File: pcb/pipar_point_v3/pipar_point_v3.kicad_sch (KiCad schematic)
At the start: 3 parts

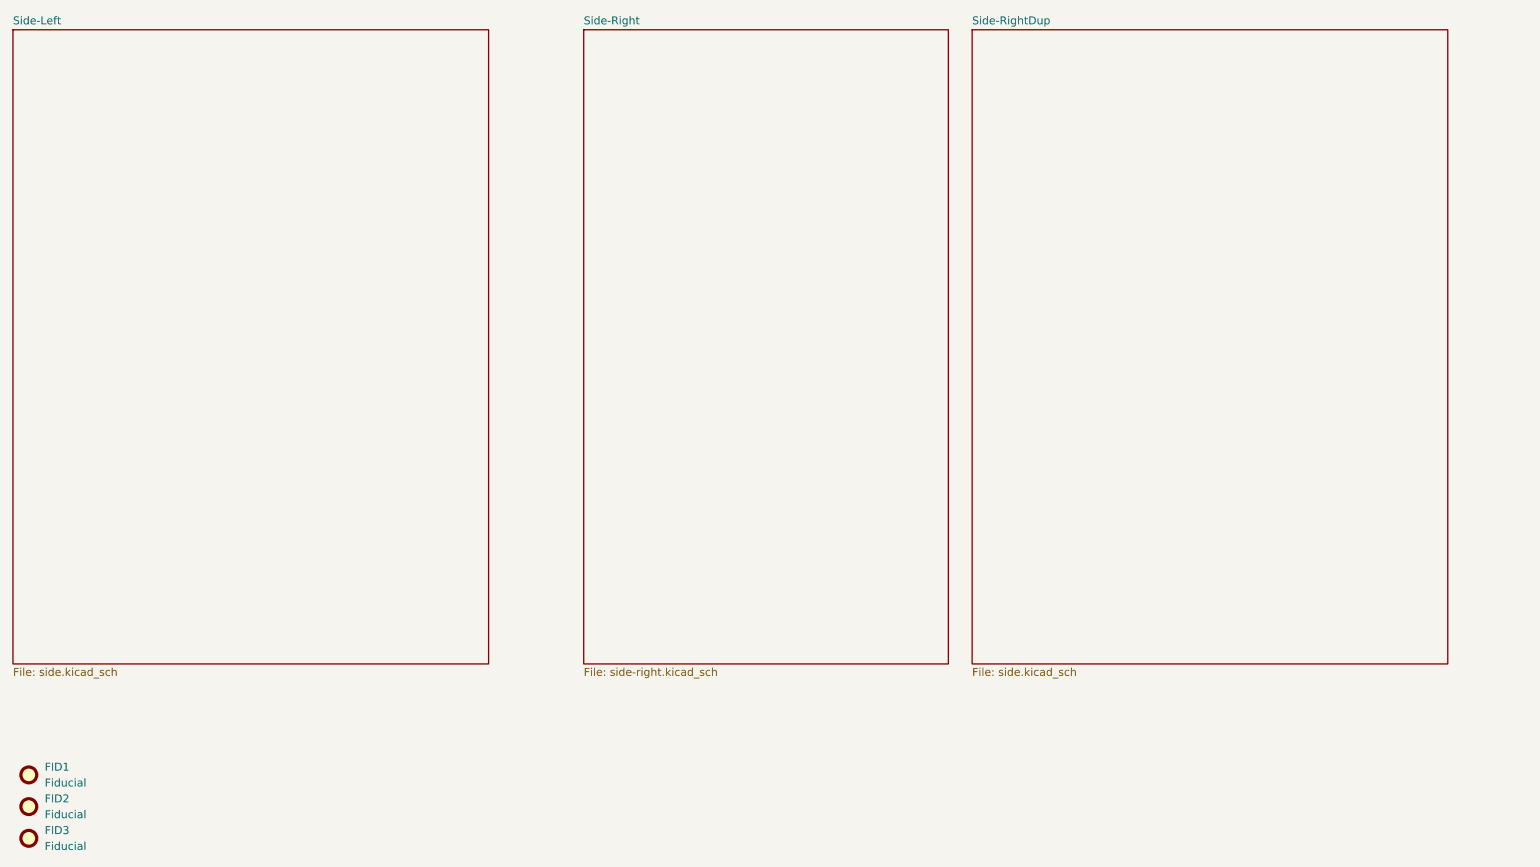
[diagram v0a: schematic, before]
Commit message: Refactor schematic connections and add hierarchical labels
- Removed redundant no_connect entries and updated UUIDs for clarity.
- Added new no_connect entries at specified coordinates.
- Introduced hierarchical labels for "3.3V", "TPClock", "TPData", and "TPRST" with appropriate formatting and positioning.
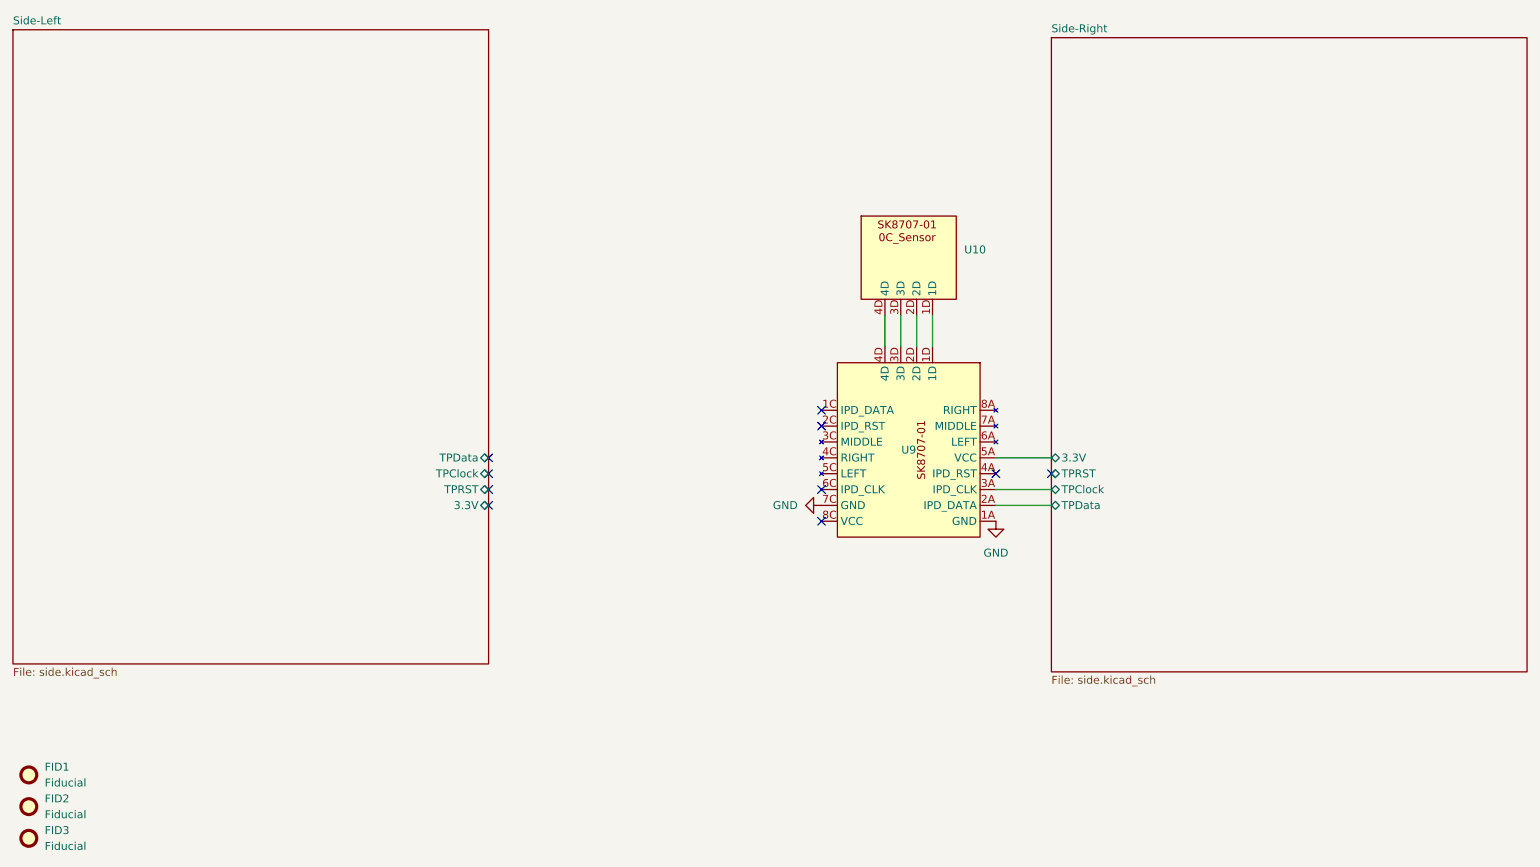
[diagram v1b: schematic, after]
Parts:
- added U10: ~, Trackpoint:SK8707-01-0C Sensor, symbol Keyboard:SK8707-01-0C_Sensor
- added U9: ~, Trackpoint:SK8707-01, symbol Keyboard:SK8707-01
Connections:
- new net: U10.1D, U9.1D
- new net: U10.2D, U9.2D
- new net: U10.3D, U9.3D
- new net: U10.4D, U9.4D
- new net GND: U9.1A (GND), U9.7C (GND)
- new net Side-Right/3.3V: U9.5A (VCC)
- new net Side-Right/TPClock: U9.3A (IPD_CLK)
- new net Side-Right/TPData: U9.2A (IPD_DATA)
- no-connect marks 0 -> 10
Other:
- removed sheet Side-RightDup
- sheet Side-Left ports: added 3.3V, TPClock, TPData, TPRST; removed none
- sheet Side-Right: file side-right.kicad_sch -> side.kicad_sch
- sheet Side-Right ports: added 3.3V, TPClock, TPData, TPRST; removed none
